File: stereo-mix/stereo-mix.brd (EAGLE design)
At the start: 149.4 x 22.4 mm, 22 parts, among them IC3 LM324N

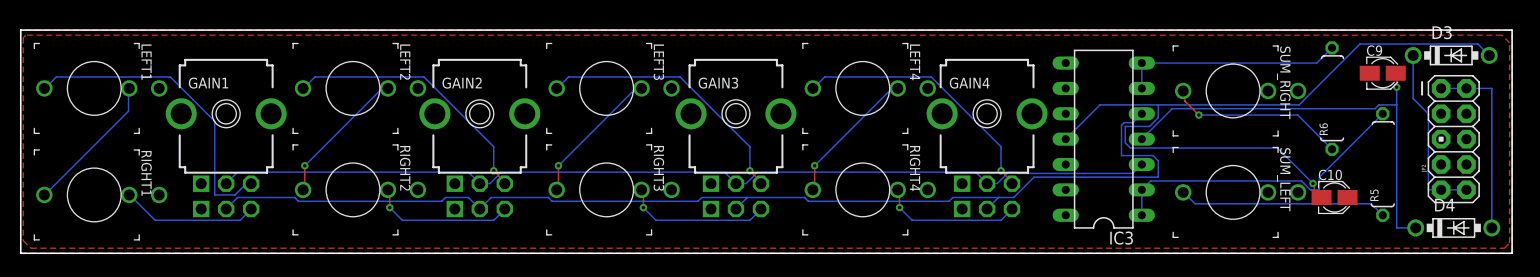
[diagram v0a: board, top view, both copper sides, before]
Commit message: gerber
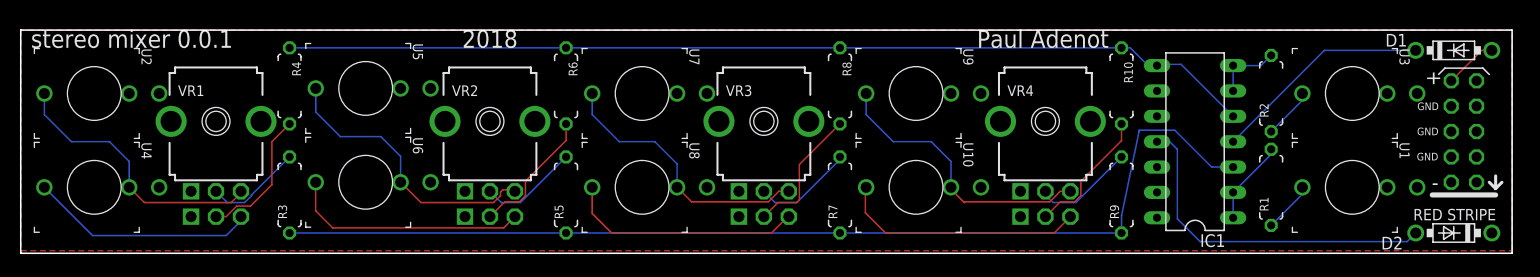
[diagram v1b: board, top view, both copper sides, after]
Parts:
- removed C10, C9: 4.7u, rcl:PANASONIC_A
- removed D3, D4: 1N5819HW, diode:DO41-7.6
- removed GAIN1, GAIN2, GAIN3, GAIN4: 10k, MusicThingModular:DUAL_9MM_SNAP-IN_POT
- removed IC3: LM324N, linear:DIL14
- removed JP2: M05X2PTH, og-header:AVR_ICSP
- removed LEFT1, LEFT2, LEFT3, LEFT4, RIGHT1, RIGHT2, RIGHT3, RIGHT4, SUM_LEFT, SUM_RIGHT: THONKICONNNEW, MusicThingModular:WQP-PJ301M-12_JACK
- added D1, D2: (no value), diode:DO41-7.6
- added IC1: (no value), linear:DIL14
- added R1, R2: 1k, MusicThingModular:7MM_RESISTOR
- added R10, R3, R4, R7, R8, R9: 100k, MusicThingModular:7MM_RESISTOR
- added SV1: EURO_POWER_HEADERREGULAR, MusicThingModular:EURO_POWER_HEADER
- added U1, U10, U2, U3, U4, U5, U6, U7, U8, U9: THONKICONNNEW, MusicThingModular:WQP-PJ301M-12_JACK
- added VR1, VR2, VR3, VR4: 10k, MusicThingModular:DUAL_9MM_SNAP-IN_POT
- R5, R6: value 1k -> 100k; device MusicThingModular:10MM_RESISTOR -> MusicThingModular:7MM_RESISTOR
- moved R5 81.8 mm to (54.6, 5.84)
- moved R6 76.7 mm to (54.6, 16.8), turned to 270 degrees
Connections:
- removed net N$23: D4.A, JP2.1, JP2.2
- removed net N$24: D3.C, JP2.10, JP2.9
- removed net N$26: LEFT1.P$2_SWITCH, RIGHT1.P$1_TIP
- removed net N$30: GAIN1.3B, RIGHT1.P$2_SWITCH
- removed net N$34: LEFT2.P$2_SWITCH, RIGHT2.P$1_TIP
- removed net N$35: GAIN2.3, LEFT2.P$1_TIP
- removed net N$36: GAIN2.3B, RIGHT2.P$2_SWITCH
- removed net N$39: LEFT3.P$2_SWITCH, RIGHT3.P$1_TIP
- removed net N$41: GAIN3.3B, RIGHT3.P$2_SWITCH
- removed net N$44: LEFT4.P$2_SWITCH, RIGHT4.P$1_TIP
- removed net N$46: GAIN4.3B, RIGHT4.P$2_SWITCH
- new net N$1: R4.2, VR1.2B
- new net N$10: D2.C, SV1.2
- new net N$11: U4.P$1_TIP, VR1.3B
- new net N$12: U5.P$1_TIP, U6.P$2_SWITCH, VR2.3
- new net N$13: U6.P$1_TIP, VR2.3B
- new net N$14: D1.A, SV1.10
- new net N$15: U8.P$1_TIP, VR3.3B
- new net N$18: U10.P$1_TIP, VR4.3B
- new net N$2: R3.2, VR1.2
- new net N$3: R5.2, VR2.2
- new net N$4: R6.2, VR2.2B
- new net N$5: R7.2, VR3.2
- new net N$7: R8.2, VR3.2B
- new net N$8: R9.2, VR4.2
- new net N$9: R10.2, VR4.2B
- net GND: now also SV1.3, SV1.5, SV1.7, U1.P$3_SLEEVE, U10.P$3_SLEEVE, U2.P$3_SLEEVE, U3.P$3_SLEEVE, U4.P$3_SLEEVE, U5.P$3_SLEEVE, U6.P$3_SLEEVE, U7.P$3_SLEEVE, U8.P$3_SLEEVE, U9.P$3_SLEEVE, VR1.1, VR1.1B, VR2.1, VR2.1B, VR3.1, VR3.1B, VR4.1, VR4.1B; no longer C10.+, C9.-, JP2.3, JP2.4, JP2.5, JP2.6, JP2.7, JP2.8, LEFT1.P$3_SLEEVE, LEFT2.P$3_SLEEVE, LEFT3.P$3_SLEEVE, LEFT4.P$3_SLEEVE, RIGHT1.P$3_SLEEVE, RIGHT2.P$3_SLEEVE, RIGHT3.P$3_SLEEVE, RIGHT4.P$3_SLEEVE, SUM_LEFT.P$3_SLEEVE, SUM_RIGHT.P$3_SLEEVE
- net N$20: now also R2.1, U3.P$1_TIP; no longer R6.1, SUM_RIGHT.P$1_TIP
- net N$25: now also U2.P$1_TIP, U4.P$2_SWITCH, VR1.3; no longer GAIN1.3, LEFT1.P$1_TIP
- net N$27: now also IC1.6, IC1.7, R2.2; no longer IC3.6, IC3.7, R6.2
- net N$29: now also IC1.1, IC1.2, R1.2; no longer IC3.1, IC3.2, R5.2
- net N$40: now also U7.P$1_TIP, U8.P$2_SWITCH, VR3.3; no longer GAIN3.3, LEFT3.P$1_TIP
- net N$45: now also U10.P$2_SWITCH, U9.P$1_TIP, VR4.3; no longer GAIN4.3, LEFT4.P$1_TIP
- net N$47: now also IC1.3, R3.1, R5.1, R7.1, R9.1; no longer GAIN1.2, GAIN2.2, GAIN3.2, GAIN4.2, IC3.3
- net N$48: now also IC1.5, R10.1, R4.1, R6.1, R8.1; no longer GAIN1.2B, GAIN2.2B, GAIN3.2B, GAIN4.2B, IC3.5
- net N$6: now also R1.1, U1.P$1_TIP; no longer R5.1, SUM_LEFT.P$1_TIP
- net VCC: now also D1.C, IC1.4; no longer C9.+, D4.C, IC3.4
- net VEE: now also D2.A, IC1.11; no longer C10.-, D3.A, IC3.11
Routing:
- net VEE: track 75.7 -> 34.5 mm, vias 1 -> 0
- net N$12: track 0.00 -> 28.4 mm
- net N$35: track 26.7 -> 0.00 mm, vias 1 -> 0
- net N$18: track 0.00 -> 24.6 mm
- net N$13: track 0.00 -> 24.0 mm
- net N$15: track 0.00 -> 23.8 mm
- net N$29: track 31.3 -> 8.44 mm
- net N$11: track 0.00 -> 22.7 mm
- net VCC: track 44.4 -> 22.1 mm, vias 1 -> 0
- net N$23: track 19.0 -> 0.00 mm
- net N$24: track 17.9 -> 0.00 mm
- net N$6: track 20.9 -> 5.11 mm
- net N$27: track 22.2 -> 6.77 mm
- net N$41: track 14.7 -> 0.00 mm, vias 1 -> 0
- net N$36: track 14.4 -> 0.00 mm, vias 1 -> 0
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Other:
- board text added: "2018"
- board text added: "Paul Adenot"
- board text added: "stereo mixer 0.0.1"
